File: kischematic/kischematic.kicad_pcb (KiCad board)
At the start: 2 copper layers, 26.7 x 50 mm, 105 parts, among them IC1 BlueNRG, IC10 128x64OLED, IC11 BALF-BRG-01D3, IC12 MAX44009, IC2 EFM32ZG108, IC3 BQ297xx, IC4 AAT3672IWO-4.2-1, IC5 TPS6223xx, IC6 MAX44009, IC8 BSD840NH6327XTSA1, IC9 MMA8653FC, J1 0, J2 Screw_Terminal_1x01, J5 Screw_Terminal_1x01, J6 Screw_Terminal_1x01, P1 CONN_01X01, P2 CONN_01X01, P3 CONN_01X01, P4 CONN_01X01, P5 CONN_01X01, P6 CONN_01X01, P7 CONN_01X01, P8 CONN_01X04, P9 CONN_01X04, SW1 SW_Push, SW2 SW_Push, U1 USB-C, U2 SWD_SPRING, U3 FT200XD, Y1 32k, Y2 16M

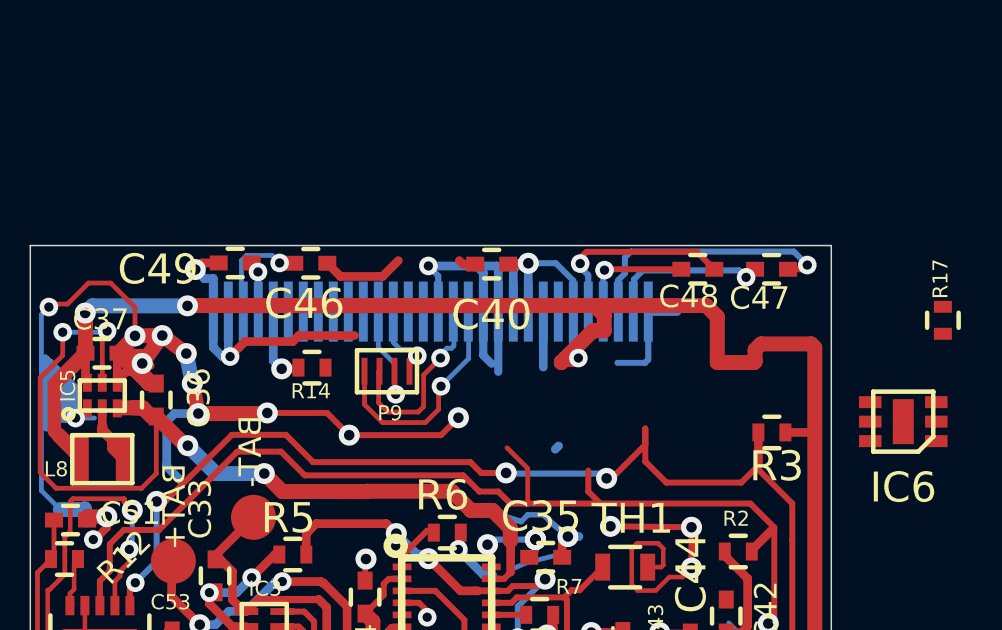
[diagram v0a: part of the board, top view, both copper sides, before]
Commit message: Tidying up.
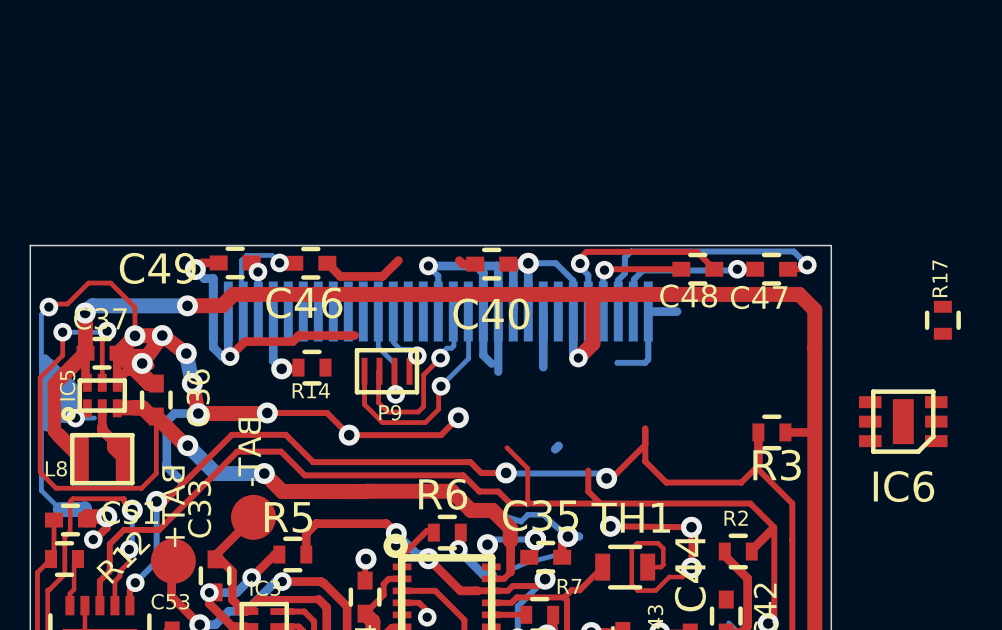
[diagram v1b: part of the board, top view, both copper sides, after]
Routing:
- net VREG: track 191.2 -> 178.7 mm
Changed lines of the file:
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@@
     (thickness 1.6)
     (drawings 223)
-    (tracks 2148)
+    (tracks 2132)
     (zones 0)
     (modules 105)
@@
   )
   (setup
-    (last_trace_width 0.1525)
+    (last_trace_width 0.5)
     (user_trace_width 0.16)
     (user_trace_width 0.2)
@@
   (segment (start 87.29 68.86) (end 87.3 68.85) (width 0.29) (layer B.Cu) (net 0))
   (segment (start 93.5 31.79) (end 93.61 31.68) (width 0.29) (layer B.Cu) (net 0))
+  (segment (start 91.1 27.2) (end 91.1 25.91) (width 0.29) (layer B.Cu) (net 1))
   (via (at 86.76 40.78) (size 0.7) (drill 0.35) (layers F.Cu B.Cu) (net 1))
   (segment (start 86.76 40.78) (end 86.94 40.96) (width 0.29) (layer F.Cu) (net 1))
@@
   (segment (start 91.6 27.2) (end 91.6 25.73) (width 0.29) (layer B.Cu) (net 1))
   (segment (start 91.1 25.91) (end 90.87 25.68) (width 0.29) (layer B.Cu) (net 1))
-  (segment (start 91.1 27.2) (end 91.1 25.91) (width 0.29) (layer B.Cu) (net 1))
   (segment (start 96.6 28.8) (end 96.49 28.91) (width 0.2) (layer B.Cu) (net 1))
   (segment (start 96.49 28.91) (end 95.57 28.91) (width 0.2) (layer B.Cu) (net 1))
@@
   (segment (start 94 47) (end 94.71 46.29) (width 0.2) (layer F.Cu) (net 1) (status 30))
   (segment (start 94 47) (end 95 48) (width 0.2) (layer F.Cu) (net 1) (status 30))
+  (segment (start 94.74 26.63) (end 94.753 26.643) (width 0.5) (layer F.Cu) (net 2))
+  (segment (start 94.753 26.643) (end 94.753 28.267) (width 0.5) (layer F.Cu) (net 2))
+  (segment (start 94.753 28.267) (end 94.27 28.75) (width 0.5) (layer F.Cu) (net 2))
+  (segment (start 82.77 26.63) (end 94.74 26.63) (width 0.5) (layer F.Cu) (net 2))
+  (segment (start 94.74 26.63) (end 101.63 26.63) (width 0.5) (layer F.Cu) (net 2))
+  (segment (start 81.24 27.01) (end 82.4 27) (width 0.5) (layer F.Cu) (net 2))
+  (segment (start 82.4 27) (end 82.77 26.63) (width 0.5) (layer F.Cu) (net 2))
+  (segment (start 101.63 26.63) (end 102.15 27.15) (width 0.5) (layer F.Cu) (net 2))
+  (segment (start 102.15 27.15) (end 102.15 28.4) (width 0.5) (layer F.Cu) (net 2))
+  (segment (start 102.15 28.4) (end 102.15 31.21) (width 0.5) (layer F.Cu) (net 2))
   (via (at 94.27 28.75) (size 0.62) (drill 0.31) (layers F.Cu B.Cu) (net 2))
-  (segment (start 94.12 28.9) (end 93.7 28.9) (width 0.29) (layer F.Cu) (net 2))
   (segment (start 96.61 42.12) (end 96.45 41.96) (width 0.42) (layer F.Cu) (net 2))
   (segment (start 96.45 41.66) (end 95.545 40.755) (width 0.42) (layer F.Cu) (net 2))
@@
   (segment (start 85.35 62.22) (end 86.5 61.07) (width 0.29) (layer F.Cu) (net 2))
   (segment (start 86.5 61.07) (end 86.5 60.75) (width 0.29) (layer F.Cu) (net 2))
-  (segment (start 100.16 28.87) (end 100.16 28.474) (width 0.5) (layer F.Cu) (net 2))
-  (segment (start 100.354 28.28) (end 102.03 28.28) (width 0.5) (layer F.Cu) (net 2))
-  (segment (start 100.16 28.474) (end 100.354 28.28) (width 0.5) (layer F.Cu) (net 2))
-  (segment (start 102.03 28.28) (end 102.15 28.4) (width 0.5) (layer F.Cu) (net 2))
-  (segment (start 102.15 28.4) (end 102.15 31.21) (width 0.5) (layer F.Cu) (net 2))
   (segment (start 92.15 42.67) (end 92.15 42.65) (width 0.5) (layer F.Cu) (net 2))
   (segment (start 88.52 68.32) (end 89.93 68.32) (width 0.2) (layer F.Cu) (net 2))
@@
   (segment (start 81.24 27.01) (end 78.07 27.01) (width 0.5) (layer B.Cu) (net 2))
   (segment (start 78.07 27.01) (end 77.83 27.25) (width 0.5) (layer B.Cu) (net 2))
-  (segment (start 89.94 27) (end 81.25 27) (width 0.5) (layer F.Cu) (net 2))
   (segment (start 81.25 27) (end 81.24 27.01) (width 0.5) (layer F.Cu) (net 2))
   (via (at 77.83 27.25) (size 0.7) (drill 0.35) (layers F.Cu B.Cu) (net 2))
@@
   (segment (start 96.537957 47.997577) (end 96.537957 48.017957) (width 0.2) (layer F.Cu) (net 2))
   (segment (start 98.18 48.45) (end 98.18 48.9) (width 0.2) (layer F.Cu) (net 2) (status 10))
-  (segment (start 94.27 28.75) (end 94.12 28.9) (width 0.29) (layer F.Cu) (net 2))
   (segment (start 94.1 27.2) (end 94.1 28.58) (width 0.29) (layer B.Cu) (net 2))
   (segment (start 94.1 28.58) (end 94.27 28.75) (width 0.29) (layer B.Cu) (net 2))
@@
   (segment (start 97.1 39.8) (end 97.475 39.8) (width 0.2) (layer F.Cu) (net 2))
   (segment (start 90.087818 46.91) (end 90.388909 47.211091) (width 0.29) (layer F.Cu) (net 2))
-  (segment (start 82.4 27) (end 89.94 27) (width 0.5) (layer F.Cu) (net 2))
-  (segment (start 92.6 26.94) (end 92.54 27) (width 0.29) (layer F.Cu) (net 2))
-  (segment (start 89.94 27) (end 92.54 27) (width 0.5) (layer F.Cu) (net 2))
-  (segment (start 89.84 26.9) (end 89.94 27) (width 0.29) (layer F.Cu) (net 2))
-  (segment (start 94.801 27) (end 98.528 27) (width 0.5) (layer F.Cu) (net 2))
-  (segment (start 89.94 27) (end 94.801 27) (width 0.5) (layer F.Cu) (net 2))
-  (segment (start 98.9 27.372) (end 98.528 27) (width 0.5) (layer F.Cu) (net 2))
-  (segment (start 95.13 27.329) (end 94.801 27) (width 0.5) (layer F.Cu) (net 2))
   (segment (start 92.57 25.62) (end 92.6 25.59) (width 0.29) (layer B.Cu) (net 2))
   (segment (start 93.52 25.59) (end 92.6 25.59) (width 0.2) (layer B.Cu) (net 2))
@@
   (segment (start 98.12 49.99) (end 98.33 50.2) (width 0.2) (layer F.Cu) (net 2) (status 30))
   (segment (start 98.18 48.9) (end 98.12 48.96) (width 0.2) (layer F.Cu) (net 2))
-  (segment (start 98.9 28.9) (end 100.13 28.9) (width 0.5) (layer F.Cu) (net 2) (status 30))
-  (segment (start 100.13 28.9) (end 100.16 28.87) (width 0.5) (layer F.Cu) (net 2) (status 30))
-  (segment (start 98.9 28.9) (end 98.9 27.372) (width 0.5) (layer F.Cu) (net 2) (status 10))
-  (segment (start 95.13 27.84) (end 95.13 27.329) (width 0.5) (layer F.Cu) (net 2) (status 10))
-  (segment (start 93.7 28.893) (end 94.753 27.84) (width 0.5) (layer F.Cu) (net 2) (status 10))
-  (segment (start 94.753 27.84) (end 95.13 27.84) (width 0.5) (layer F.Cu) (net 2) (status 20))
-  (segment (start 93.7 28.9) (end 93.7 28.893) (width 0.5) (layer F.Cu) (net 2) (status 30))
   (segment (start 94.1 27.2) (end 94.1 26.17) (width 0.2) (layer B.Cu) (net 2) (status 10))
   (segment (start 92.6 27.2) (end 92.6 25.59) (width 0.29) (layer B.Cu) (net 2) (status 10))
@@
   (via (at 86.5 65.75) (size 0.7) (drill 0.35) (layers F.Cu B.Cu) (net 2))
   (segment (start 79.05 65.25) (end 79.28 65.02) (width 0.25) (layer F.Cu) (net 2))
-  (segment (start 93.7 28.9) (end 93.7 28.92) (width 0.2) (layer F.Cu) (net 2) (status 30))
-  (segment (start 94 28.6) (end 93.7 28.9) (width 0.5) (layer F.Cu) (net 2) (status 30))
   (segment (start 77.84 28.59) (end 76.94 29.49) (width 0.5) (layer F.Cu) (net 2) (status 10))
   (segment (start 76.94 31.315) (end 77.675 32.05) (width 0.5) (layer F.Cu) (net 2) (status 20))
@@
   (segment (start 101.76 25.79) (end 101.9 25.65) (width 0.2) (layer F.Cu) (net 71))
   (via (at 101.9 25.65) (size 0.62) (drill 0.31) (layers F.Cu B.Cu) (net 71))
-  (segment (start 99.86 26.06) (end 99.63 25.83) (width 0.2) (layer B.Cu) (net 72))
-  (segment (start 99.63 25.83) (end 96.42 25.83) (width 0.2) (layer B.Cu) (net 72))
+  (via (at 99.57 25.79) (size 0.62) (drill 0.31) (layers F.Cu B.Cu) (net 72))
+  (segment (start 99.57 25.79) (end 99.53 25.83) (width 0.2) (layer B.Cu) (net 72))
+  (segment (start 99.53 25.83) (end 96.42 25.83) (width 0.2) (layer B.Cu) (net 72))
   (segment (start 96.42 25.83) (end 96.13 26.12) (width 0.2) (layer B.Cu) (net 72))
-  (segment (start 96.13 26.12) (end 96.13 27.17) (width 0.2) (layer B.Cu) (net 72) (status 20))
+  (segment (start 96.13 26.12) (end 96.13 27.17) (width 0.2) (layer B.Cu) (net 72))
+  (segment (start 99.57 25.79) (end 100.16 25.79) (width 0.16) (layer F.Cu) (net 72))
   (segment (start 96.13 27.17) (end 96.1 27.2) (width 0.16) (layer B.Cu) (net 72) (status 30))
-  (segment (start 100.16 25.79) (end 100.13 25.79) (width 0.16) (layer F.Cu) (net 72) (status 30))
-  (segment (start 100.13 25.79) (end 99.86 26.06) (width 0.16) (layer F.Cu) (net 72) (status 10))
-  (via (at 99.86 26.06) (size 0.62) (drill 0.31) (layers F.Cu B.Cu) (net 72))
   (segment (start 83.38 25.67) (end 83.38 25.58) (width 0.29) (layer F.Cu) (net 73) (status 30))
   (segment (start 83.59 25.88) (end 83.38 25.67) (width 0.29) (layer F.Cu) (net 73) (status 20))
